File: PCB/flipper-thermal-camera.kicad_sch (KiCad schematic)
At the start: 19 parts, among them IC1 VEML7700-TT, J1 Conn_01x08, J2 Conn_01x10, U1 MLX90640ESF-BAB-000-SP, U2 XC6206PxxxMR, U3 ICM-20948, U4 SHT31-DIS

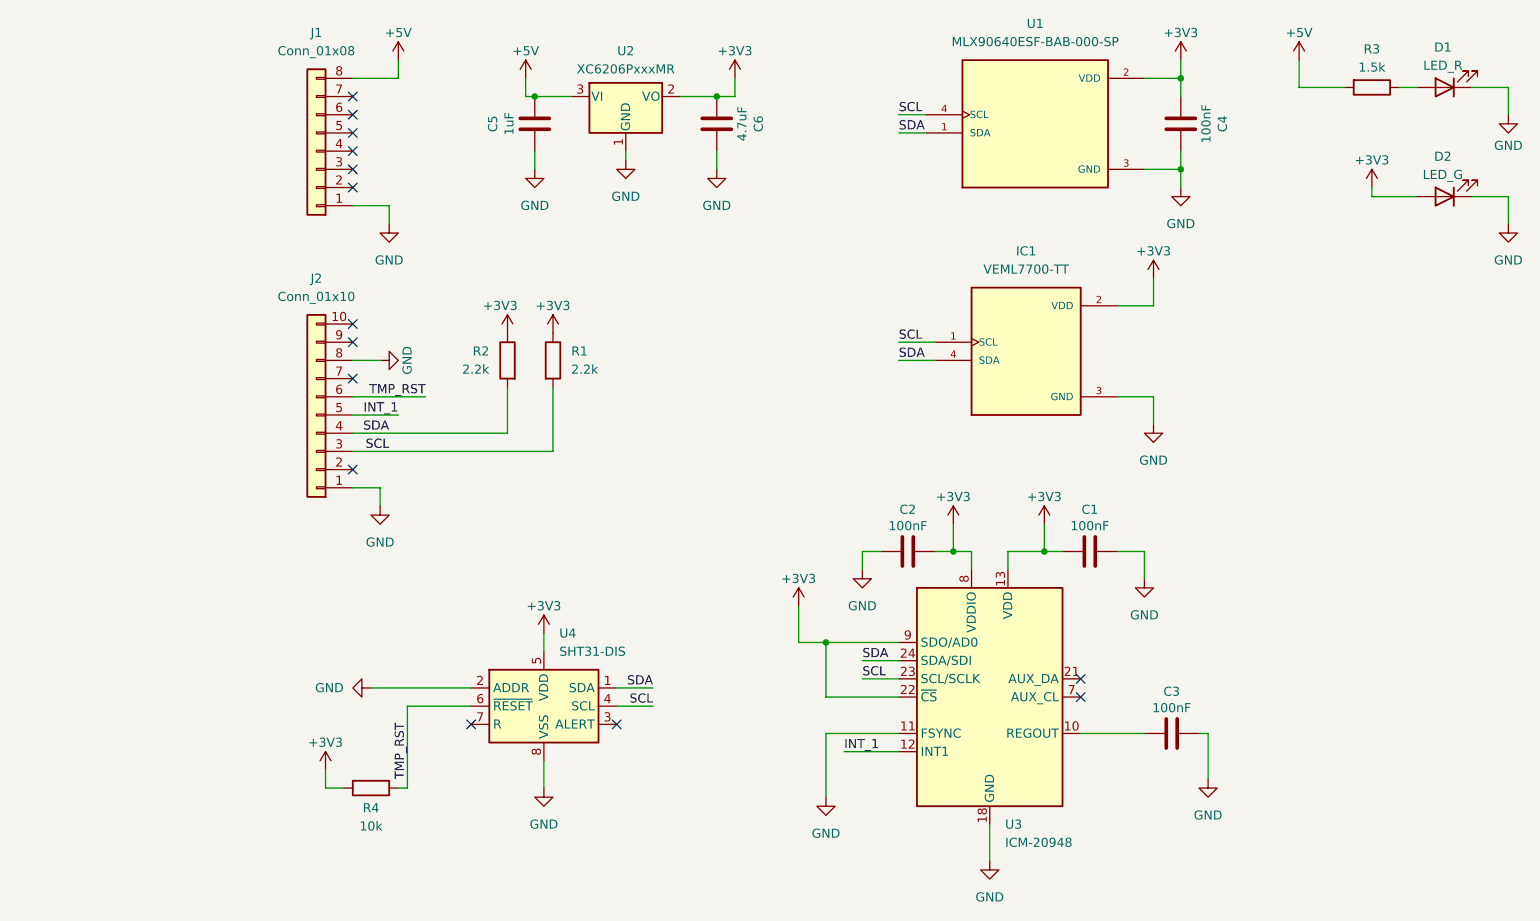
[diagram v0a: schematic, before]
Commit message: finish routing pcb
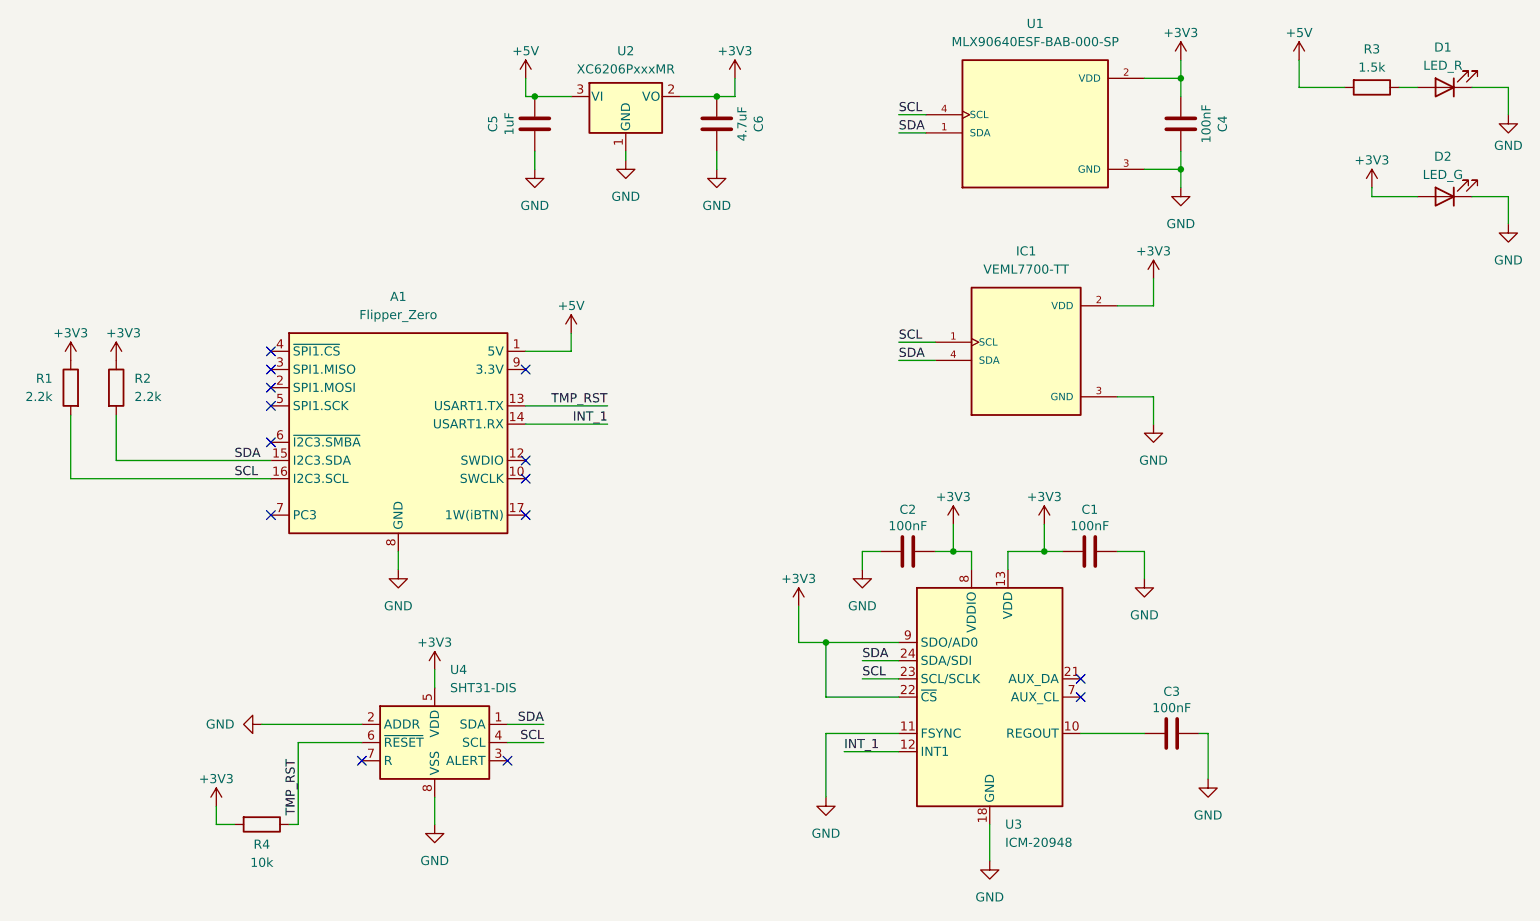
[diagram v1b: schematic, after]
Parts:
- removed J1: Conn_01x08, Connector_PinHeader_2.54mm:PinHeader_1x08_P2.54mm_Horizontal, symbol Connector_Generic:Conn_01x08
- removed J2: Conn_01x10, Connector_PinHeader_2.54mm:PinHeader_1x10_P2.54mm_Horizontal, symbol Connector_Generic:Conn_01x10
- added A1: Flipper_Zero, Module:Flipper_Zero_Angled, symbol MCU_Module:Flipper_Zero
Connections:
- net +5V: now also A1.1 (5V)
- net GND: now also A1.11 (GND), A1.18 (GND), A1.8 (GND)
- net INT_1: now also A1.14 (USART1.RX)
- net SCL: now also A1.16 (I2C3.SCL)
- net SDA: now also A1.15 (I2C3.SDA)
- net TMP_RST: now also A1.13 (USART1.TX)
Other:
- moved on the sheet: R4, U4
